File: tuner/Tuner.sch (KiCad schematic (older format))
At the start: 6 parts, among them J1 SUPP28, P1 CONN_01X03, U1 LM324

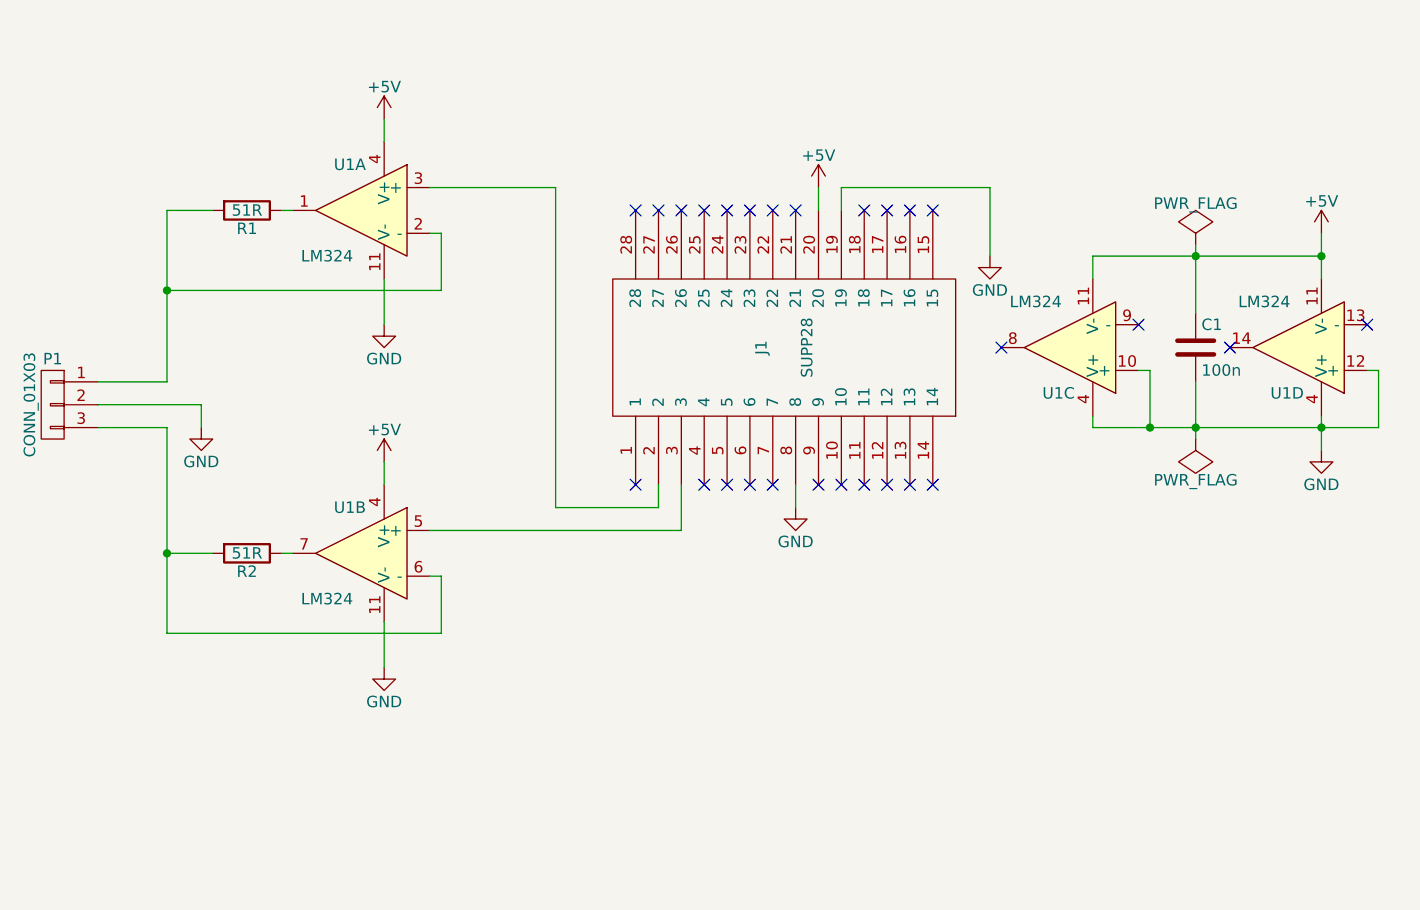
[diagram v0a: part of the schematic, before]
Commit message: kicad schematics
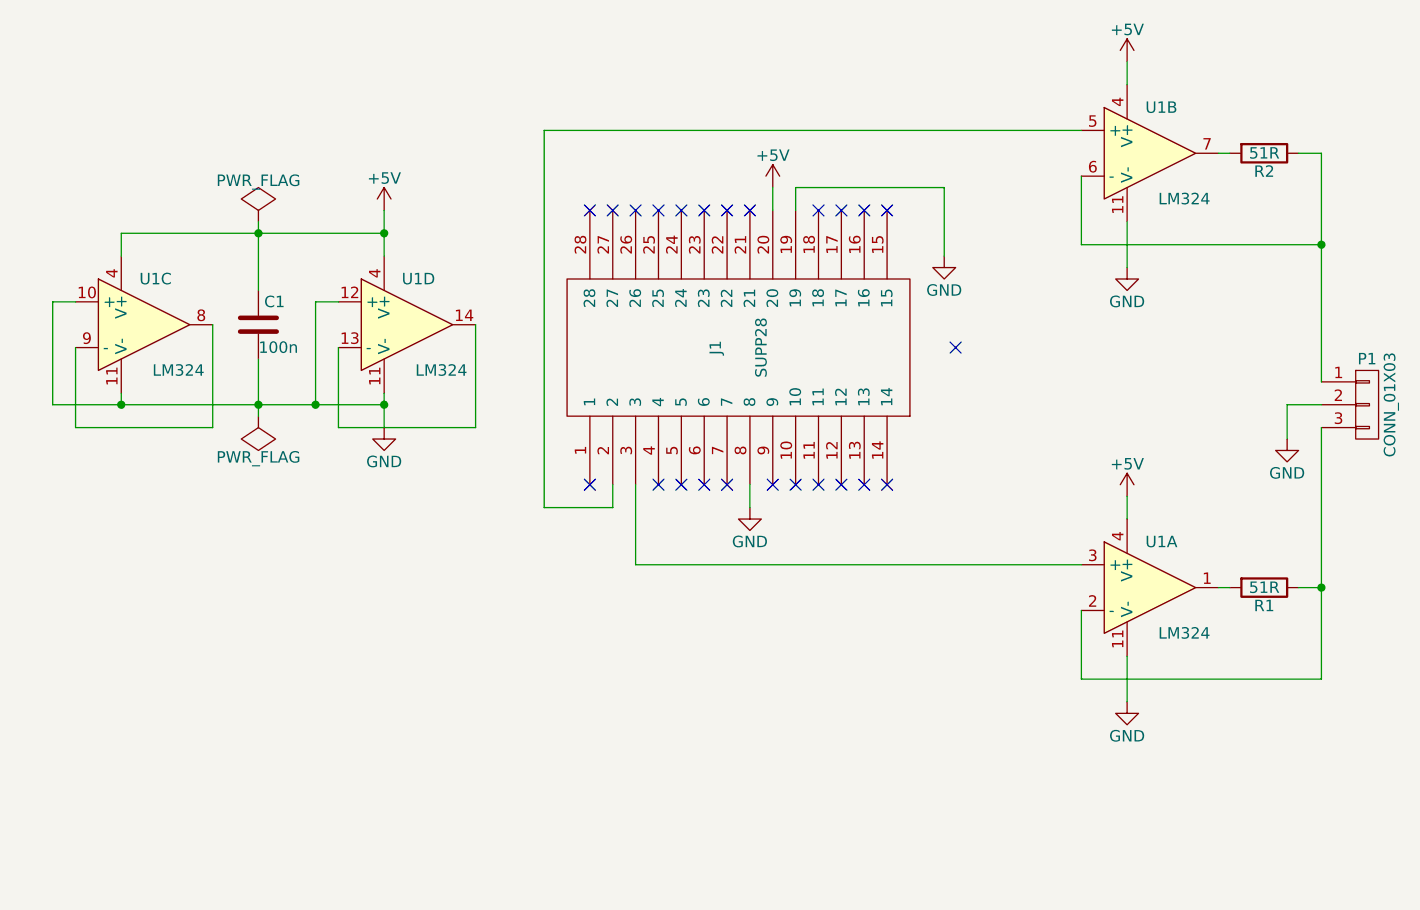
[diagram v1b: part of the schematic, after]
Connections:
- net +5V: now also U1.4 (V+), U1.4 (V+); no longer U1.11 (V-), U1.11 (V-)
- net GND: now also U1.11 (V-), U1.11 (V-); no longer U1.4 (V+), U1.4 (V+)
- net at U1.5 (+): now also J1.2; no longer J1.3
- net at R2.1: now also P1.1 (P1), U1.6 (-); no longer U1.7
- net at U1.13 (-): now also U1.14
- net at U1.8: now also U1.9 (-)
- net at U1.1: now also R1.2; no longer R1.1
- net at U1.3 (+): now also J1.3; no longer J1.2
- new net: R2.2, U1.7
- new net: P1.3 (P3), R1.1, U1.2 (-)
- no-connect marks 27 -> 24
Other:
- moved on the sheet: C1, J1, P1, R1, R2, U1A, U1B, U1C, U1D
